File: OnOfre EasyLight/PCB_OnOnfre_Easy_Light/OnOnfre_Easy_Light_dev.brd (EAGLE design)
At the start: 44.6 x 48 mm, 38 parts, among them J3Y S8050, K1 OMRON-G3MB-202P-SSR2, K2 OMRON-G3MB-202P-SSR2, U2 esp12, X1 4P

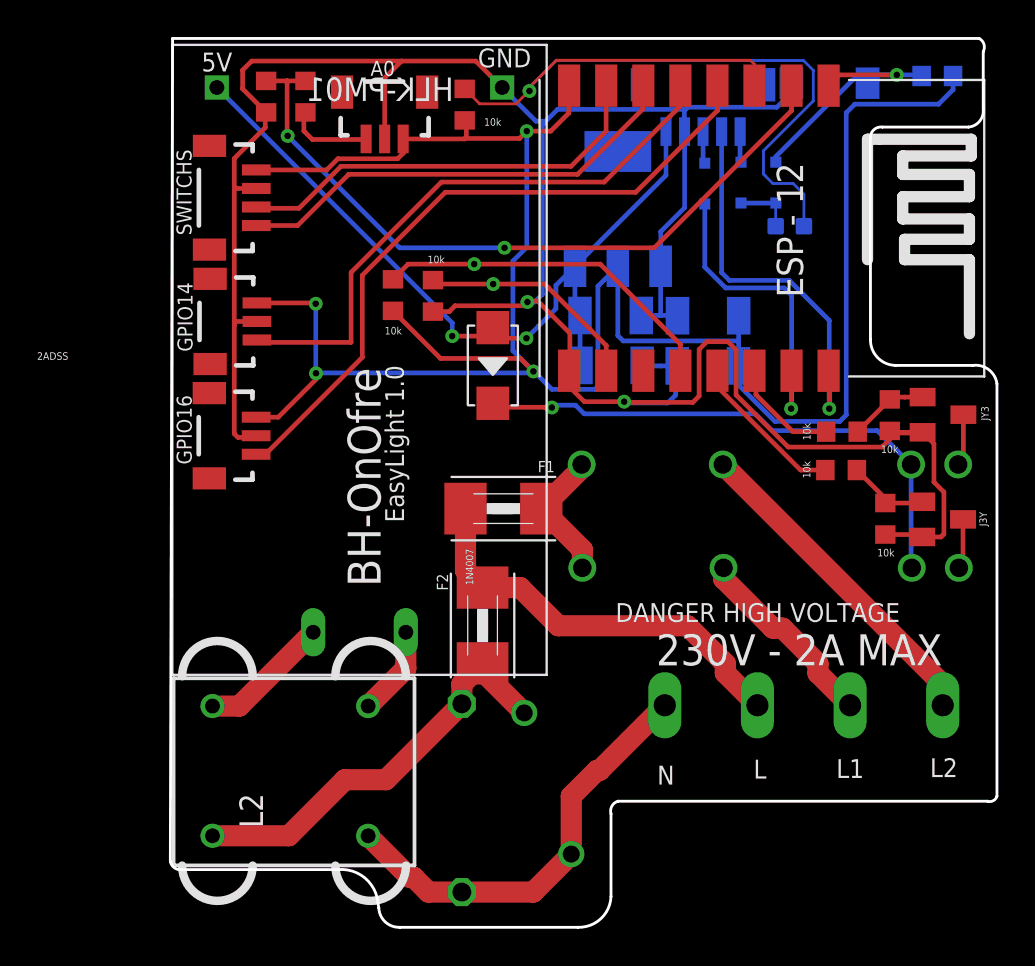
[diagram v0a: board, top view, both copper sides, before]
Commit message: easy light board
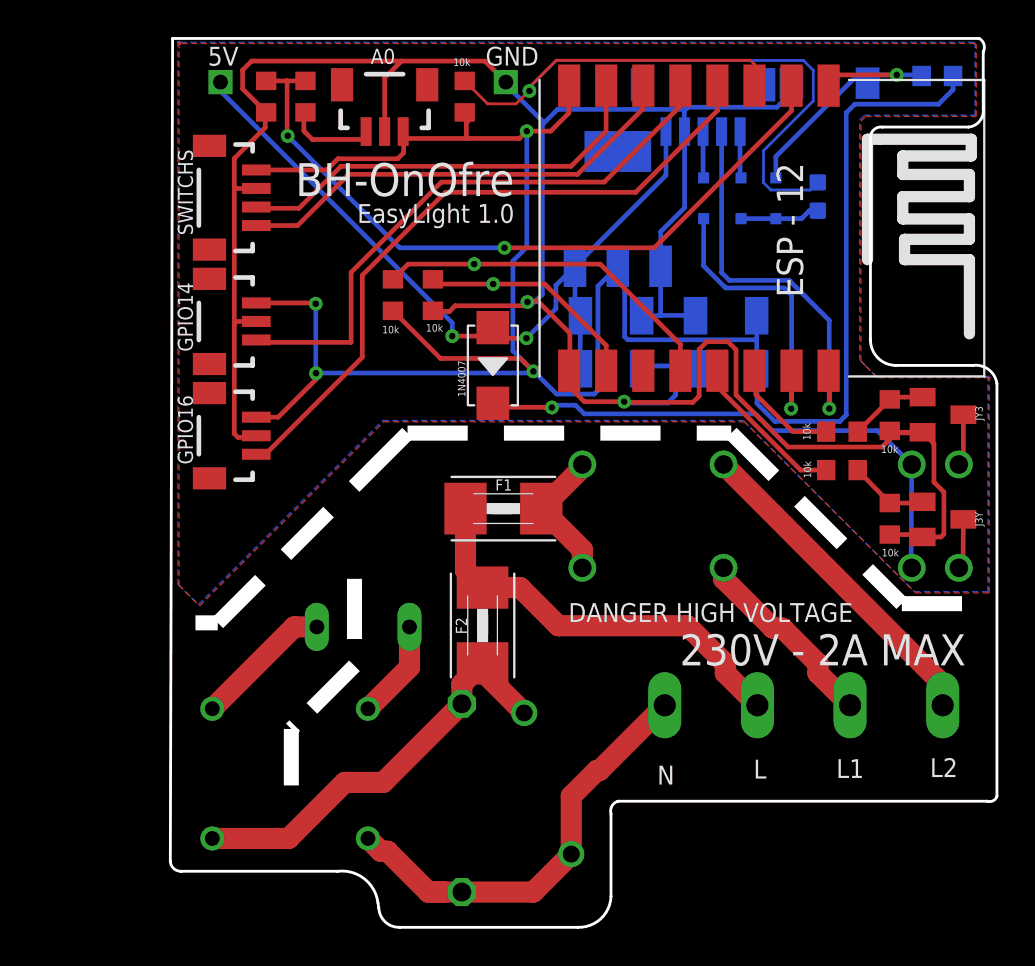
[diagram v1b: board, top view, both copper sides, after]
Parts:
- moved L2 9.85 mm to (13.4, 11.9), flipped to the bottom, turned to 270 degrees
- moved C6 2.20 mm to (35.2, 38.0), turned to 0 degrees
- moved C1 1.00 mm to (30.2, 28.7)
- moved C4 0.97 mm to (30.2, 31.6)
- moved D4 0.85 mm to (32.9, 37.9)
- moved D2 0.84 mm to (31.0, 37.9)
- moved D1 0.79 mm to (29.0, 37.9)
- moved R9 0.43 mm to (16.1, 43.4)
- moved A0 0.40 mm to (11.8, 43.1)
- moved U$2 0.35 mm to (10.6, 29.5), flipped to the top
- moved R3 0.24 mm to (39.1, 20.6)
- moved C2 0.19 mm to (24.0, 28.7)
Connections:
- net EMI_LIVE: now also L2.1, U$2.P$1; no longer L2.4, U$2.P$2
- net EMI_NEUTRAL: now also L2.2, U$2.P$2; no longer L2.3, U$2.P$1
- net GND: now also U$2.P$4; no longer U$2.P$3
- net N$2: now also L2.4; no longer L2.1
- net NEUTRAL: now also L2.3; no longer L2.2
- net VCC_1: now also U$2.P$3; no longer U$2.P$4
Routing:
- net GND: track 140.8 -> 142.3 mm
- net VCC_2: track 122.4 -> 123.7 mm
- net N$4: track 3.14 -> 4.37 mm
- net RESET: track 14.6 -> 15.4 mm
- net DTR: track 1.68 -> 2.51 mm
- net NEUTRAL: track 23.3 -> 24.1 mm
- net N$3: track 1.75 -> 2.51 mm
- net RX: track 16.9 -> 16.1 mm
- net EMI_NEUTRAL: track 4.83 -> 5.35 mm
- added copper zone on layer 1, net GND
- added copper zone on layer 16, net GND
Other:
- outline, holes or cut-outs redrawn
- board text removed: "2ADSS"
